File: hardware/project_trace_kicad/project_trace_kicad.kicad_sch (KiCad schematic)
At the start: 0 parts

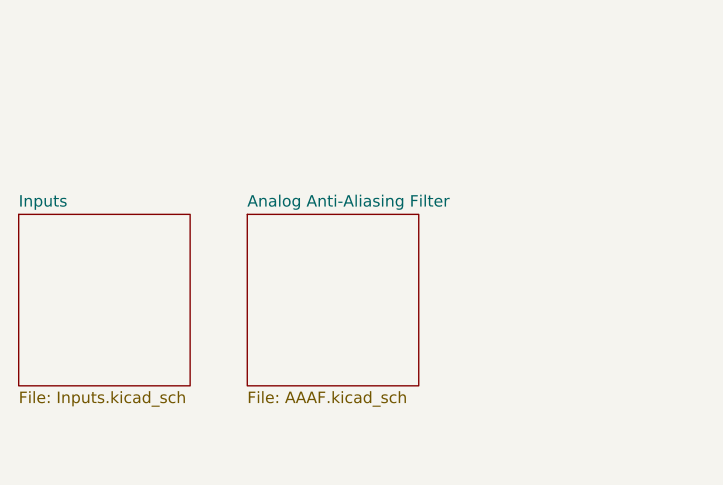
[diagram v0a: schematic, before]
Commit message: Rushed Push Footprint Lib
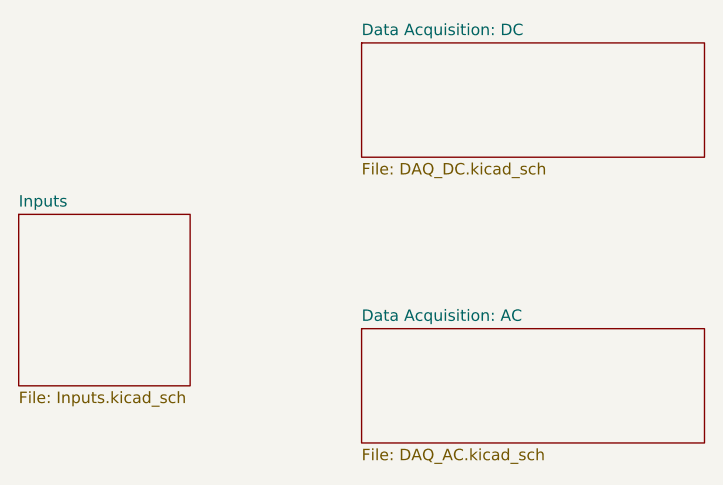
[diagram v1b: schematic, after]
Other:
- removed sheet Analog Anti-Aliasing Filter
- added sheet Data Acquisition: AC (DAQ_AC.kicad_sch)
- added sheet Data Acquisition: DC (DAQ_DC.kicad_sch)
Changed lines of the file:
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@@
 	(paper "A4")
+	(sheet
+		(at 95.25 50.8)
+		(size 38.1 12.7)
+		(exclude_from_sim no)
+		(in_bom yes)
+		(on_board yes)
+		(dnp no)
+		(fields_autoplaced yes)
+		(stroke
+			(width 0.1524)
+			(type solid)
+			(color 0 0 0 0.6)
+		)
+		(fill
+			(color 215 236 255 1.0000)
+		)
+		(property "Sheetname" "Data Acquisition: DC"
+			(at 95.25 50.0884 0)
+			(effects
+				(font
+					(size 1.27 1.27)
+				)
+				(justify left bottom)
+			)
+		)
+		(property "Sheetfile" "DAQ_DC.kicad_sch"
+			(at 95.25 64.0846 0)
+			(effects
+				(font
+					(size 1.27 1.27)
+				)
+				(justify left top)
+			)
+		)
+		(instances
+			(project "project_trace_kicad"
+				(path "/af51f4e5-b952-4b0e-baf2-78a72fb86fcd"
+					(page "4")
+				)
+			)
+		)
+	)
 	(sheet
 		(at 57.15 69.85)
@@
 	)
 	(sheet
-		(at 82.55 69.85)
-		(size 19.05 19.05)
+		(at 95.25 82.55)
+		(size 38.1 12.7)
 		(exclude_from_sim no)
 		(in_bom yes)
@@
 			(color 215 236 255 1.0000)
 		)
-		(property "Sheetname" "Analog Anti-Aliasing Filter"
-			(at 82.55 69.1384 0)
+		(property "Sheetname" "Data Acquisition: AC"
+			(at 95.25 81.8384 0)
 			(effects
 				(font
@@
 			)
 		)
-		(property "Sheetfile" "AAAF.kicad_sch"
-			(at 82.55 89.4846 0)
+		(property "Sheetfile" "DAQ_AC.kicad_sch"
+			(at 95.25 95.8346 0)
 			(effects
 				(font
